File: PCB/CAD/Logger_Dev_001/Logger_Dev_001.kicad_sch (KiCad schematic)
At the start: 4 parts, among them U2 ESP32-C6-WROOM-1

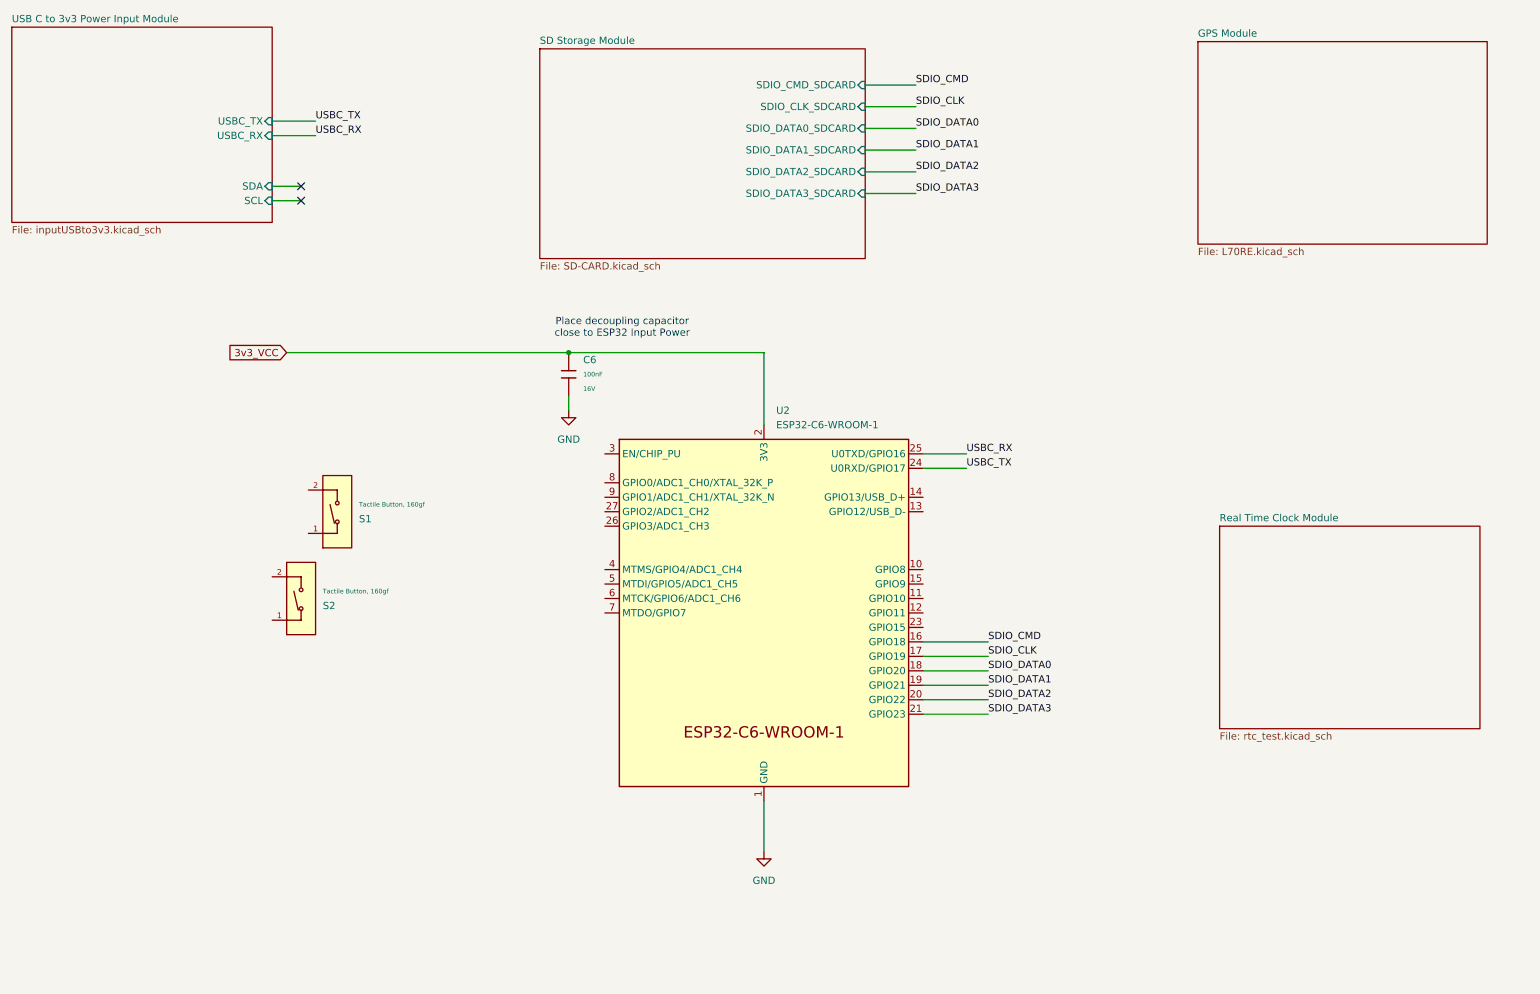
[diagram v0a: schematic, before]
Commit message: Updated Schematic
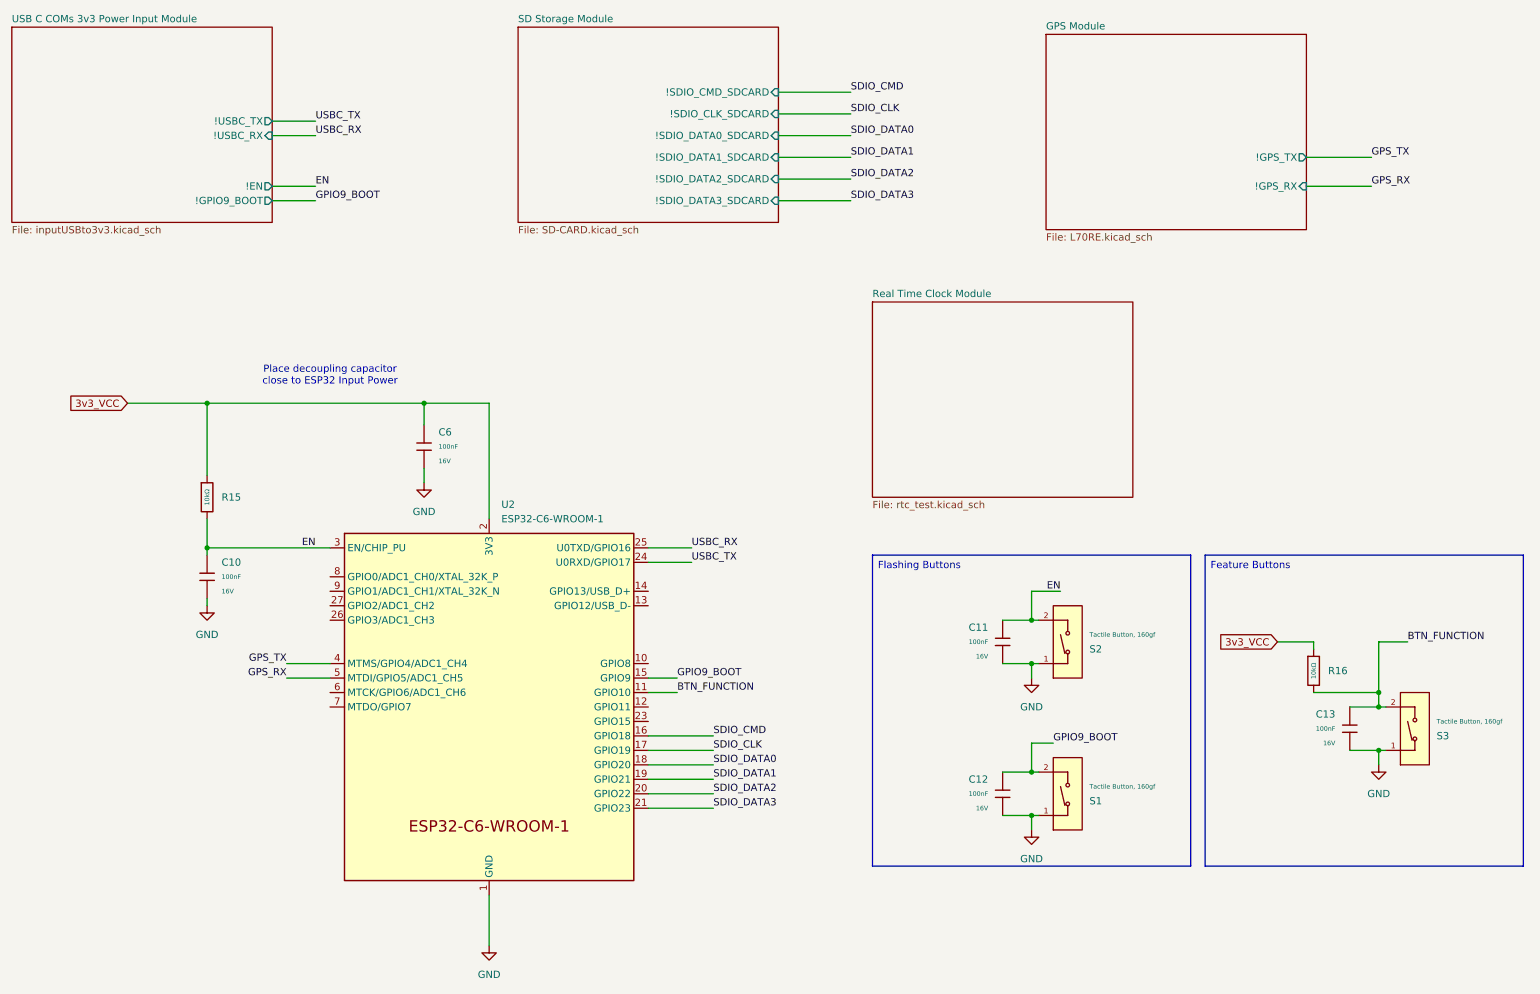
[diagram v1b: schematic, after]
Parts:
- added C10, C11, C12, C13: 100nF, PCM_JLCPCB:C_0402, symbol PCM_JLCPCB-Capacitors:0402,100nF
- added R15, R16: 10kΩ, PCM_JLCPCB:R_0402, symbol PCM_JLCPCB-Resistors:0402,10kΩ
- added S3: Tactile Button, 160gf, PCM_JLCPCB:SW_TS-1088-AR02016, symbol PCM_JLCPCB-Connectors_Buttons:Tactile Button, 160gf, 12V, 50mA, 4.0mm
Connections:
- net 3v3_VCC: now also R15.1, R16.1
- net GND: now also S1.1 (A), S2.1 (A), C10.2, C11.2, C12.2, C13.2, S3.1 (A)
- net BTN_FUNCTION: now reaches U2.11 (GPIO10)
- net BTN_FUNCTION: now also C13.1, R16.2, S3.2 (B)
- net GPIO9_BOOT: now reaches U2.15 (GPIO9)
- net GPIO9_BOOT: now also S1.2 (B), C12.1
- net EN: now reaches U2.3 (EN/CHIP_PU)
- net EN: now also S2.2 (B), C10.1, C11.1, R15.2
- net GPS_TX: now reaches U2.4 (MTMS/GPIO4/ADC1_CH4)
- net GPS_RX: now reaches U2.5 (MTDI/GPIO5/ADC1_CH5)
- no-connect marks 2 -> 0
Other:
- sheet USB C to 3v3 Power Input Module renamed USB C COMs 3v3 Power Input Module
- sheet GPS Module ports: added !GPS_RX, !GPS_TX; removed none
- sheet SD Storage Module ports: added !SDIO_CLK_SDCARD, !SDIO_CMD_SDCARD, !SDIO_DATA0_SDCARD, !SDIO_DATA1_SDCARD, !SDIO_DATA2_SDCARD, !SDIO_DATA3_SDCARD; removed SDIO_CLK_SDCARD, SDIO_CMD_SDCARD, SDIO_DATA0_SDCARD, SDIO_DATA1_SDCARD, SDIO_DATA2_SDCARD, SDIO_DATA3_SDCARD
- sheet USB C COMs 3v3 Power Input Module ports: added !EN, !GPIO9_BOOT, !USBC_RX, !USBC_TX; removed SCL, SDA, USBC_RX, USBC_TX
- company: (none) -> Jake Odgers
- title: (none) -> Mileage Logger
- moved on the sheet: C6, S1, S2, U2
